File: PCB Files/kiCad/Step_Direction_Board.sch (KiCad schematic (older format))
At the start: 3 parts, among them J0 Conn_01x02

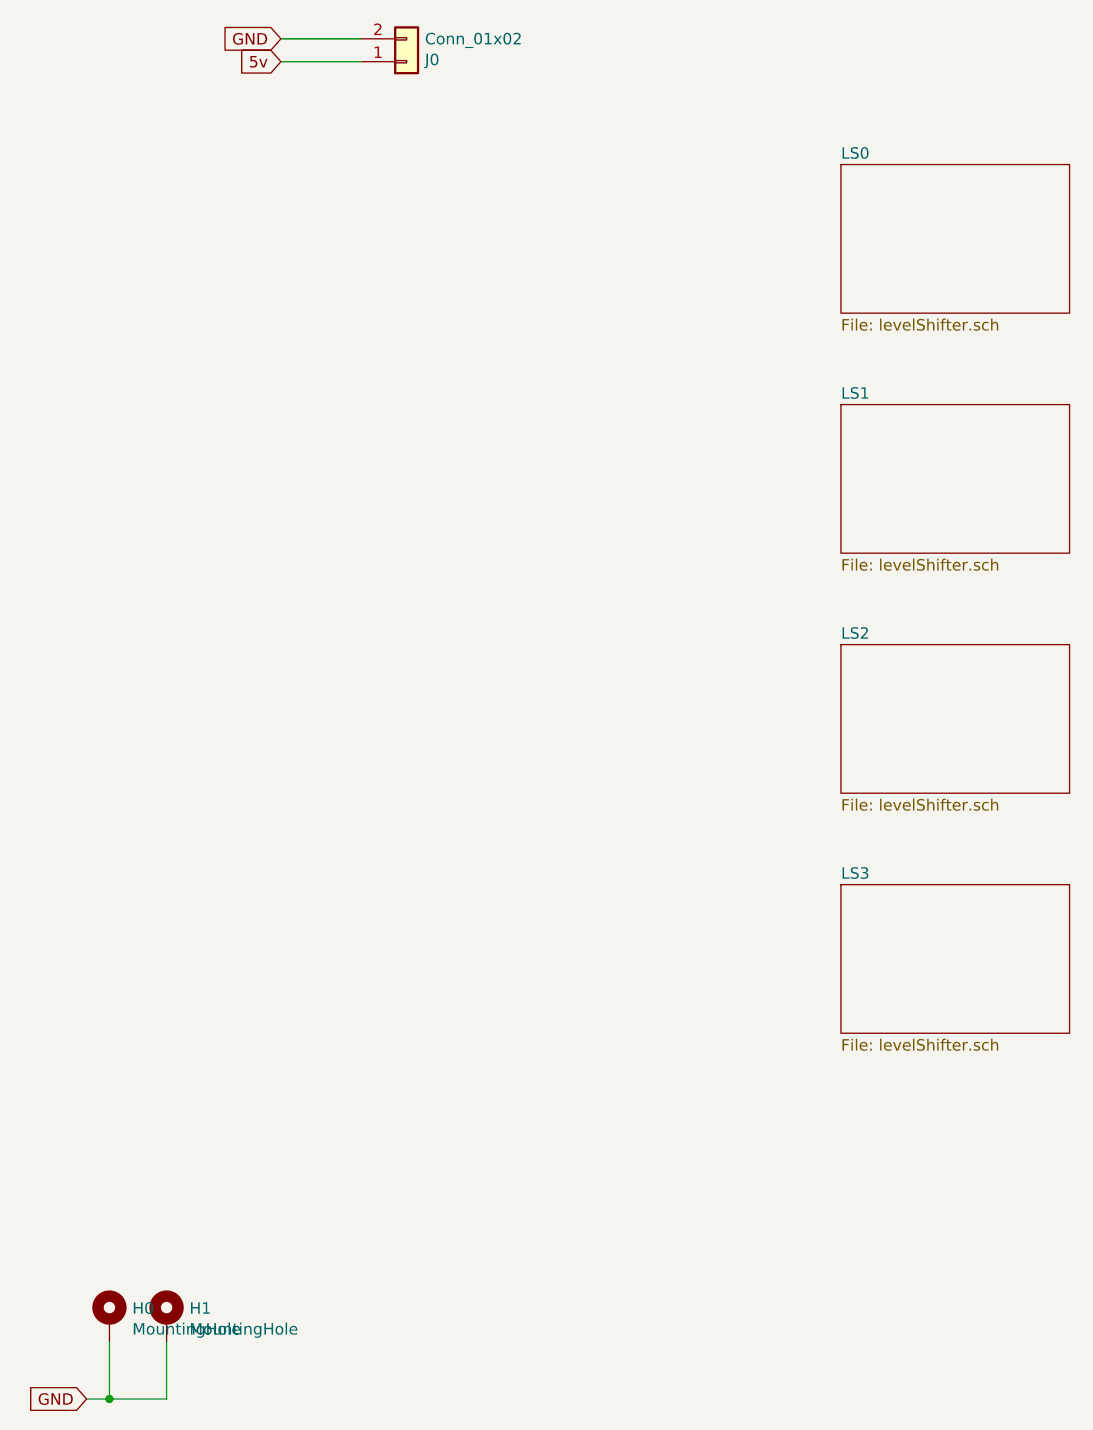
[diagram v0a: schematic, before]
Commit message: let's try this again
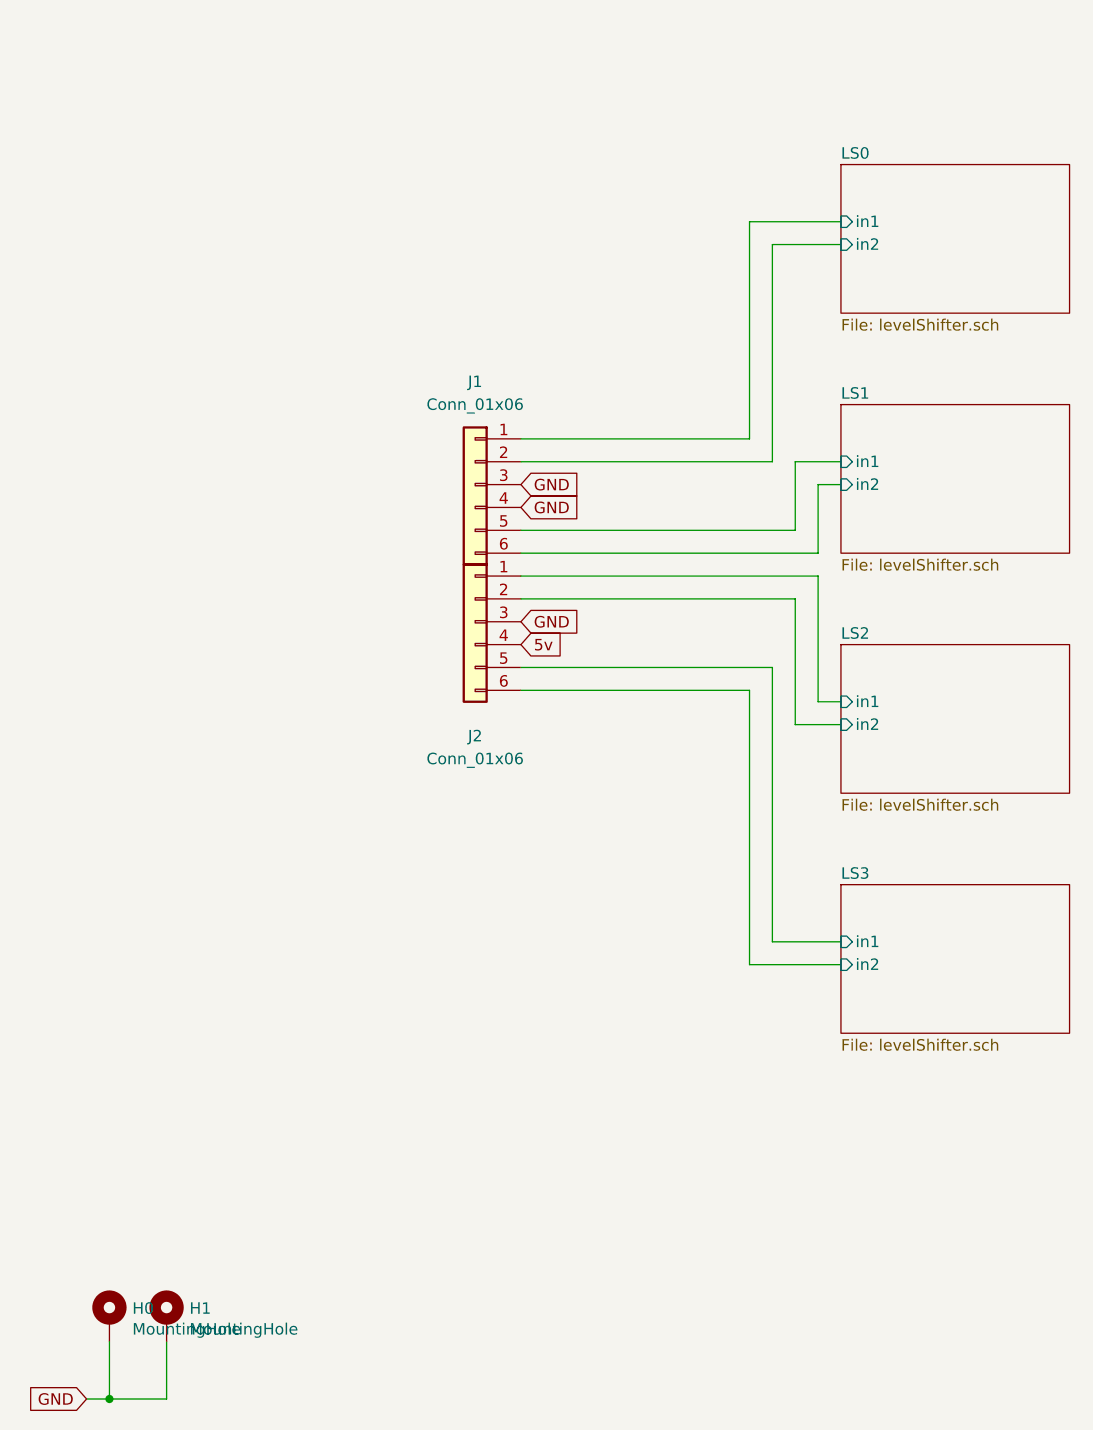
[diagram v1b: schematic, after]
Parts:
- removed J0: Conn_01x02, Connector_PinHeader_2.54mm:PinHeader_1x02_P2.54mm_Horizontal, symbol Connector_Generic:Conn_01x02
- added J1, J2: Conn_01x06, Connector_PinHeader_2.54mm:PinHeader_1x06_P2.54mm_Horizontal, symbol Connector_Generic:Conn_01x06
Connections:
- net 5v: now also J2.4 (Pin_4)
- net GND: now also J1.3 (Pin_3), J1.4 (Pin_4), J2.3 (Pin_3)
- new net LS0/in1: J1.1 (Pin_1)
- new net LS0/in2: J1.2 (Pin_2)
- new net LS1/in1: J1.5 (Pin_5)
- new net LS1/in2: J1.6 (Pin_6)
- new net LS2/in1: J2.1 (Pin_1)
- new net LS2/in2: J2.2 (Pin_2)
- new net LS3/in1: J2.5 (Pin_5)
- new net LS3/in2: J2.6 (Pin_6)
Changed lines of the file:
@@
 F0 "LS0" 50
 F1 "levelShifter.sch" 50
+F2 "in1" I L 5000 2000 50
+F3 "in2" I L 5000 2100 50
 $EndSheet
-Text GLabel 2550 1200 0    50   Input ~ 0
+Text GLabel 3600 3750 2    50   Input ~ 0
 GND
-Wire Wire Line
-	2550 1200 2900 1200
-Text GLabel 2550 1300 0    50   Input ~ 0
+Text GLabel 3600 3850 2    50   Input ~ 0
 5v
-Wire Wire Line
-	2550 1300 2900 1300
 $Sheet
 S 5000 2800 1000 650
@@
 F0 "LS1" 50
 F1 "levelShifter.sch" 50
+F2 "in1" I L 5000 3050 50
+F3 "in2" I L 5000 3150 50
 $EndSheet
 $Sheet
@@
 F0 "LS2" 50
 F1 "levelShifter.sch" 50
+F2 "in1" I L 5000 4100 50
+F3 "in2" I L 5000 4200 50
 $EndSheet
 $Sheet
@@
 F0 "LS3" 50
 F1 "levelShifter.sch" 50
+F2 "in1" I L 5000 5150 50
+F3 "in2" I L 5000 5250 50
 $EndSheet
 $Comp
@@
 	1    0    0    -1
 $EndComp
-$Comp
-L Connector_Generic:Conn_01x02 J0
-U 1 1 5E611C9B
-P 3100 1300
-F 0 "J0" H 3180 1292 50  0000 L CNN
-F 1 "Conn_01x02" H 3180 1201 50  0000 L CNN
-F 2 "Connector_PinHeader_2.54mm:PinHeader_1x02_P2.54mm_Horizontal" H 3100 1300 50  0001 C CNN
-F 3 "~" H 3100 1300 50  0001 C CNN
-	1    3100 1300
-	1    0    0    1
-$EndComp
 Text GLabel 1700 7150 0    50   Input ~ 0
 GND
@@
 	2050 7150 1800 7150
 Connection ~ 1800 7150
+Wire Wire Line
+	4600 2000 5000 2000
+Wire Wire Line
+	5000 2100 4700 2100
+Wire Wire Line
+	4700 2100 4700 3050
+Wire Wire Line
+	5000 3050 4800 3050
+Wire Wire Line
+	4800 3050 4800 3350
+Wire Wire Line
+	3600 3350 4800 3350
+Wire Wire Line
+	5000 3150 4900 3150
+Wire Wire Line
+	4900 3150 4900 3450
+Wire Wire Line
+	4900 3450 3600 3450
+Wire Wire Line
+	3600 3550 4900 3550
+Wire Wire Line
+	4900 3550 4900 4100
+Wire Wire Line
+	4900 4100 5000 4100
+Wire Wire Line
+	4800 4200 4800 3650
+Wire Wire Line
+	4800 3650 3600 3650
+Wire Wire Line
+	4800 4200 5000 4200
+Wire Wire Line
+	4700 5150 5000 5150
+Wire Wire Line
+	5000 5250 4600 5250
+Wire Wire Line
+	4600 5250 4600 4050
+$Comp
+L Connector_Generic:Conn_01x06 J2
+U 1 1 5E707B0B
+P 3400 3750
+F 0 "J2" H 3400 3250 50  0000 C CNN
+F 1 "Conn_01x06" H 3400 3150 50  0000 C CNN
+F 2 "Connector_PinHeader_2.54mm:PinHeader_1x06_P2.54mm_Horizontal" H 3400 3750 50  0001 C CNN
+F 3 "~" H 3400 3750 50  0001 C CNN
+	1    3400 3750
+	-1   0    0    -1
+$EndComp
+Text GLabel 3600 3250 2    50   Input ~ 0
+GND
+Wire Wire Line
+	3600 3950 4700 3950
+Wire Wire Line
+	4700 3950 4700 5150
+Wire Wire Line
+	3600 4050 4600 4050
+$Comp
+L Connector_Generic:Conn_01x06 J1
+U 1 1 5E70E42C
+P 3400 3150
+F 0 "J1" H 3400 3600 50  0000 C CNN
+F 1 "Conn_01x06" H 3400 3500 50  0000 C CNN
+F 2 "Connector_PinHeader_2.54mm:PinHeader_1x06_P2.54mm_Horizontal" H 3400 3150 50  0001 C CNN
+F 3 "~" H 3400 3150 50  0001 C CNN
+	1    3400 3150
+	-1   0    0    -1
+$EndComp
+Wire Wire Line
+	3600 2950 4600 2950
+Wire Wire Line
+	4600 2950 4600 2000
+Wire Wire Line
+	3600 3050 4700 3050
+Text GLabel 3600 3150 2    50   Input ~ 0
+GND
 $EndSCHEMATC
